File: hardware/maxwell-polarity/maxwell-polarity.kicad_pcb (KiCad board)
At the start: 2 copper layers, 17.8 x 17.8 mm, 5 parts, among them J1 Battery, J2 Output, SW1 SW_Push, U1 STT3P2UH7

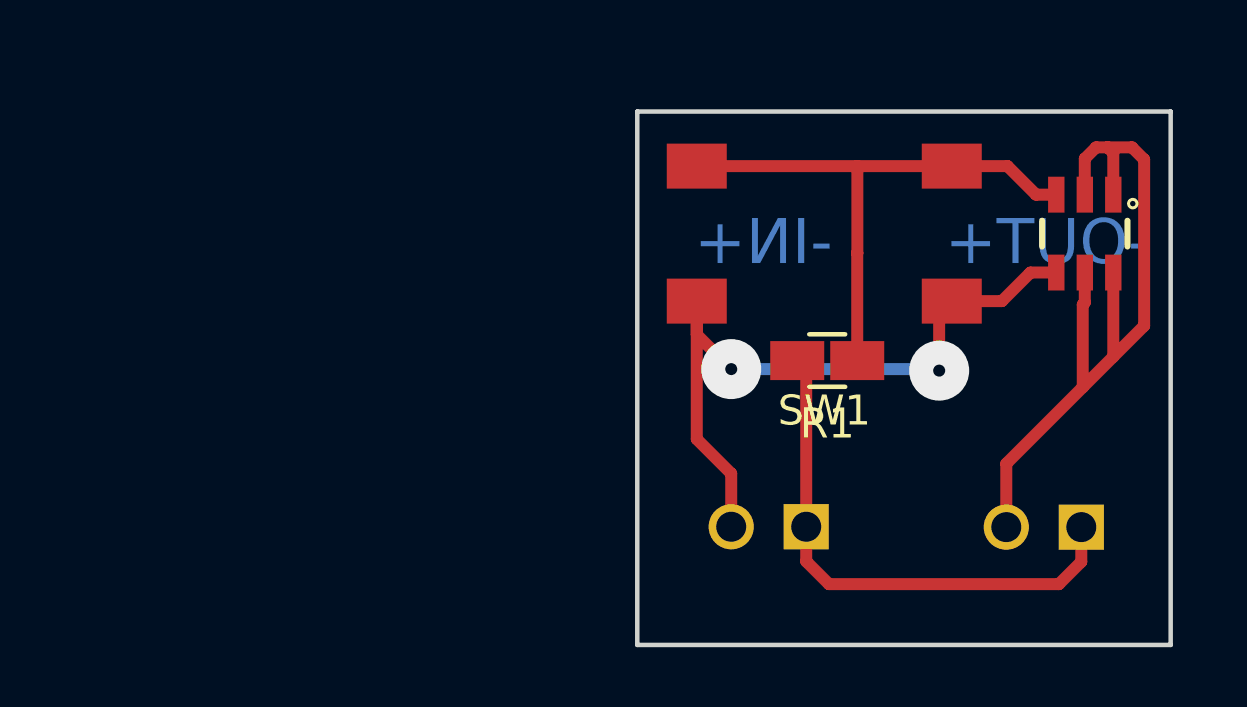
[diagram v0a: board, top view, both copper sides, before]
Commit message: Updating hardware files.
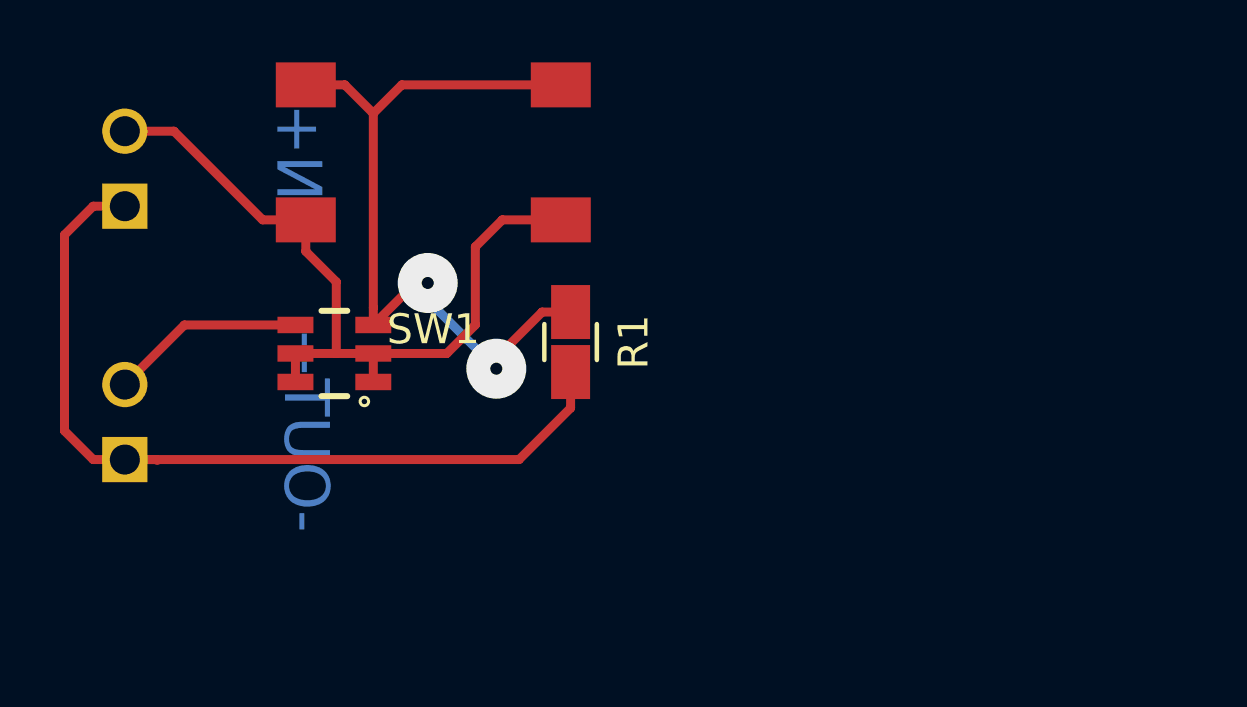
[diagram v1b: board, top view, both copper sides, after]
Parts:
- J1: value Battery -> Output
- J2: value Output -> Battery
- moved J2 32.9 mm to (129.0, 85.7), turned to 270 degrees
- moved U1 25.3 mm to (136.0, 91.9), turned to 90 degrees
- moved J1 21.7 mm to (129.0, 94.2), turned to 270 degrees
- moved SW1 13.3 mm to (139.3, 85.2)
- moved R1 8.58 mm to (143.8, 91.5), turned to 270 degrees
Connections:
- SW1 pad 2: Net-(J1-Pad2) -> Net-(J2-Pad2)
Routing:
- net Net-(J1-Pad2): track 24.1 -> 6.51 mm, vias 2 -> 0
- net GND: track 17.8 -> 29.2 mm
- net Net-(R1-Pad1): track 18.9 -> 26.0 mm, vias 0 -> 2
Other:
- board outline removed
- net class Default: clearance 0.3 -> 0.195; trace_width 0.4 -> 0.3
- rule trace_clearance: 0.3 -> 0.195
